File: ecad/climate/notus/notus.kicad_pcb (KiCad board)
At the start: 2 copper layers, 120 x 120 mm, 12 parts, among them J1 6410-02A, J2 6410-02A

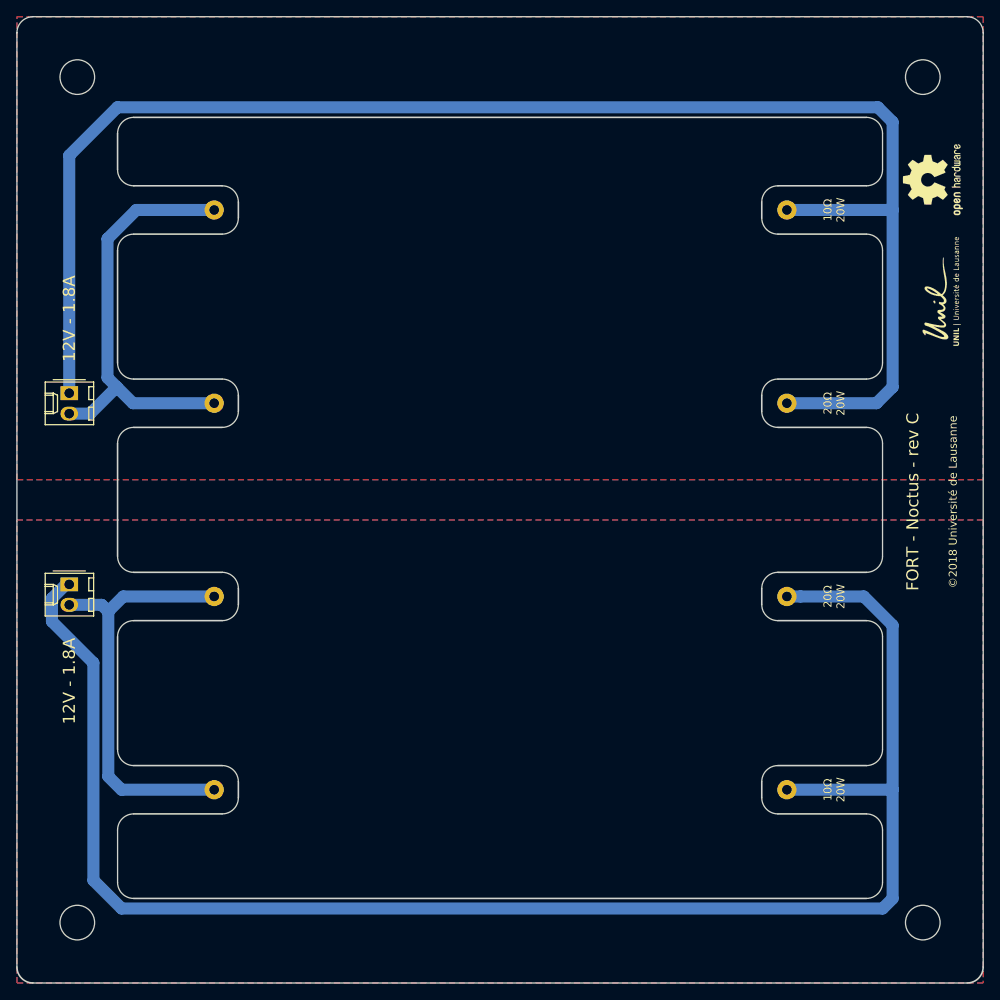
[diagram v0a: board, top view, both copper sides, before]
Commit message: Starts a brand new notus
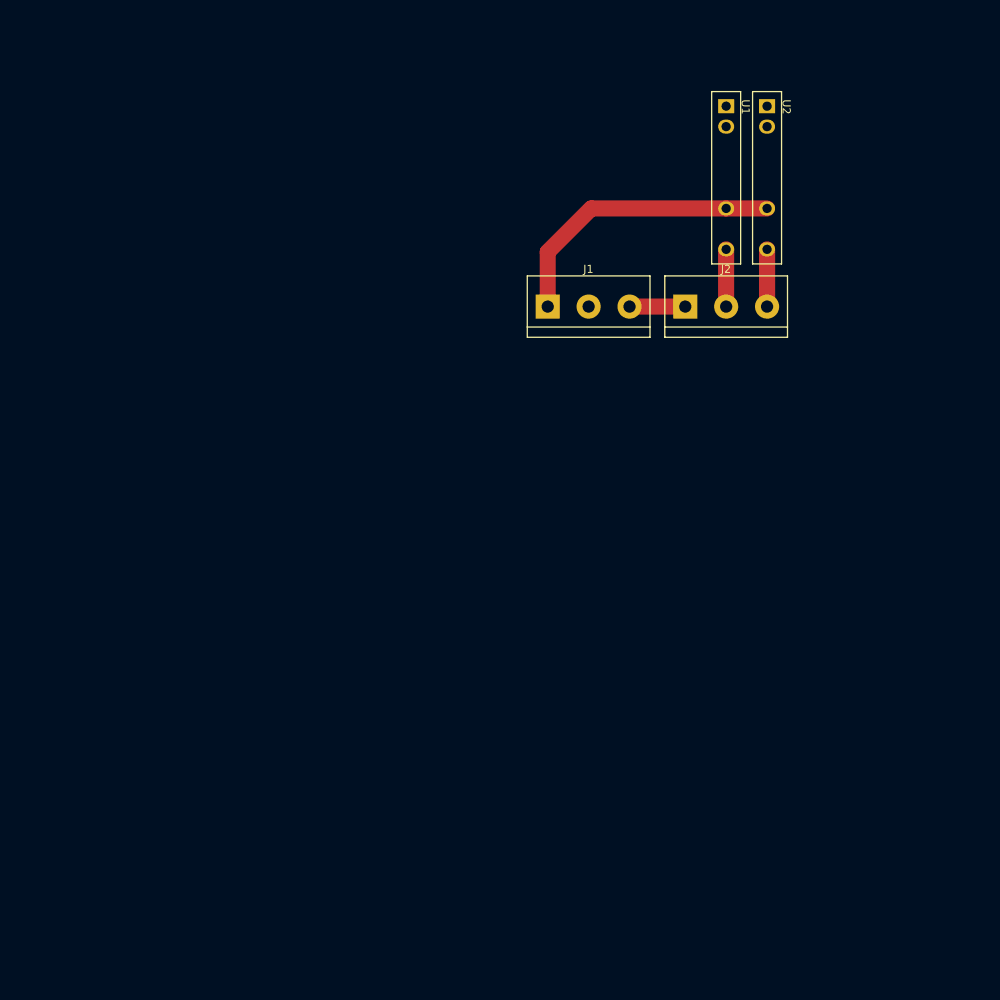
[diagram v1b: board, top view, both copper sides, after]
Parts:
- removed G***: LOGO, FORT:UNIL-LOGO_13.8x5.1mm
- removed MH1, MH2, MH3, MH4: MountingHole, MountingHole:MountingHole_4.3mm_M4_DIN965
- removed R1, R4: 10R, 20W, Resistor_THT:R_Axial_Power_L60.0mm_W14.0mm_P71.12mm
- removed R2, R3: 20R, 20W, Resistor_THT:R_Axial_Power_L60.0mm_W14.0mm_P71.12mm
- removed REF**: OSHW-Logo2_9.8x8mm_SilkScreen, Symbol:OSHW-Logo2_9.8x8mm_SilkScreen
- added U1: CPC1966YX6, FORT:SIP4_LittleFuse_CPC19X6yX6, F.Cu at (178.1, 50.0)
- added U2: CPC1966YX6, FORT:SIP4_LittleFuse_CPC19X6yX6, F.Cu at (183.2, 50.0)
- J1, J2: value 6410-02A -> Screw_Terminal_01x03; footprint Connector_Molex:Molex_KK-254_AE-6410-02A_1x02_P2.54mm_Vertical -> TerminalBlock:TerminalBlock_bornier-3_P5.08mm
- moved J2 77.3 mm to (173.0, 66.0), turned to 0 degrees
- moved J1 68.7 mm to (155.9, 66.0), turned to 0 degrees
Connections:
- J1 pad 1: /PWM_A -> /AC_L
- J1 pad 2: GND -> Earth
- J2 pad 1: /PWM_B -> /AC_N
- J2 pad 2: GNDA -> /AC_L1
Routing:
- net /PWM_A: track 202.9 -> 0.00 mm
- net /PWM_B: track 195.0 -> 0.00 mm
- net GNDA: track 53.8 -> 0.00 mm
- net GND: track 53.4 -> 0.00 mm
- net /AC_L: track 0.00 -> 36.3 mm
- net /AC_L2: track 0.00 -> 7.11 mm
- net /AC_L1: track 0.00 -> 7.11 mm
- net /AC_N: track 0.00 -> 6.92 mm
- removed copper zone on B.Cu, net GND
- removed copper zone on F.Cu, net GND
- removed copper zone on B.Cu, net GNDA
- removed copper zone on F.Cu, net GNDA
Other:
- board outline removed
- net class Default removed
- board text removed: "10Ω 20W"
- board text removed: "12V - 1.8A"
- board text removed: "20Ω 20W"
- board text removed: "FORT - Noctus - rev C"
- board text removed: "©2018 Université de Lausanne"
